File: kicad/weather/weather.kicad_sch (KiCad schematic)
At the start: 6 parts

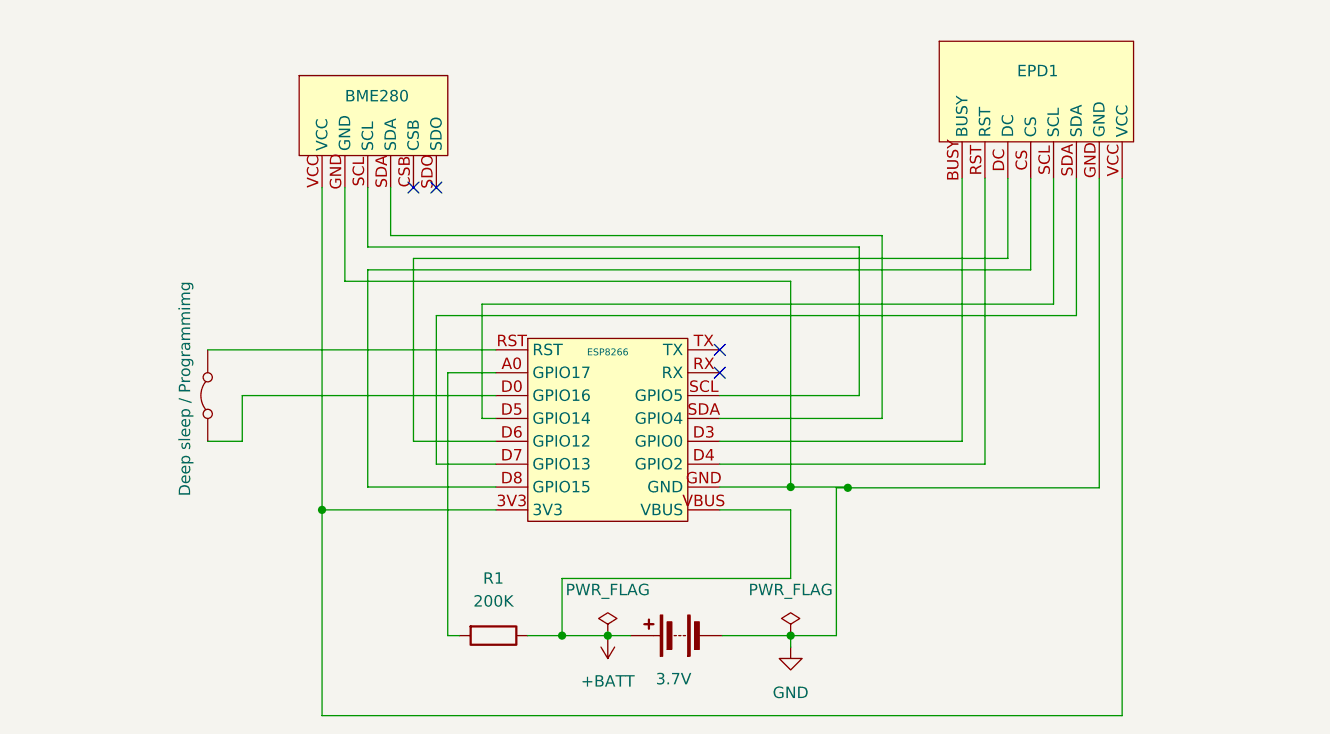
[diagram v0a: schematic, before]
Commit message: Finalized schematics and PCB
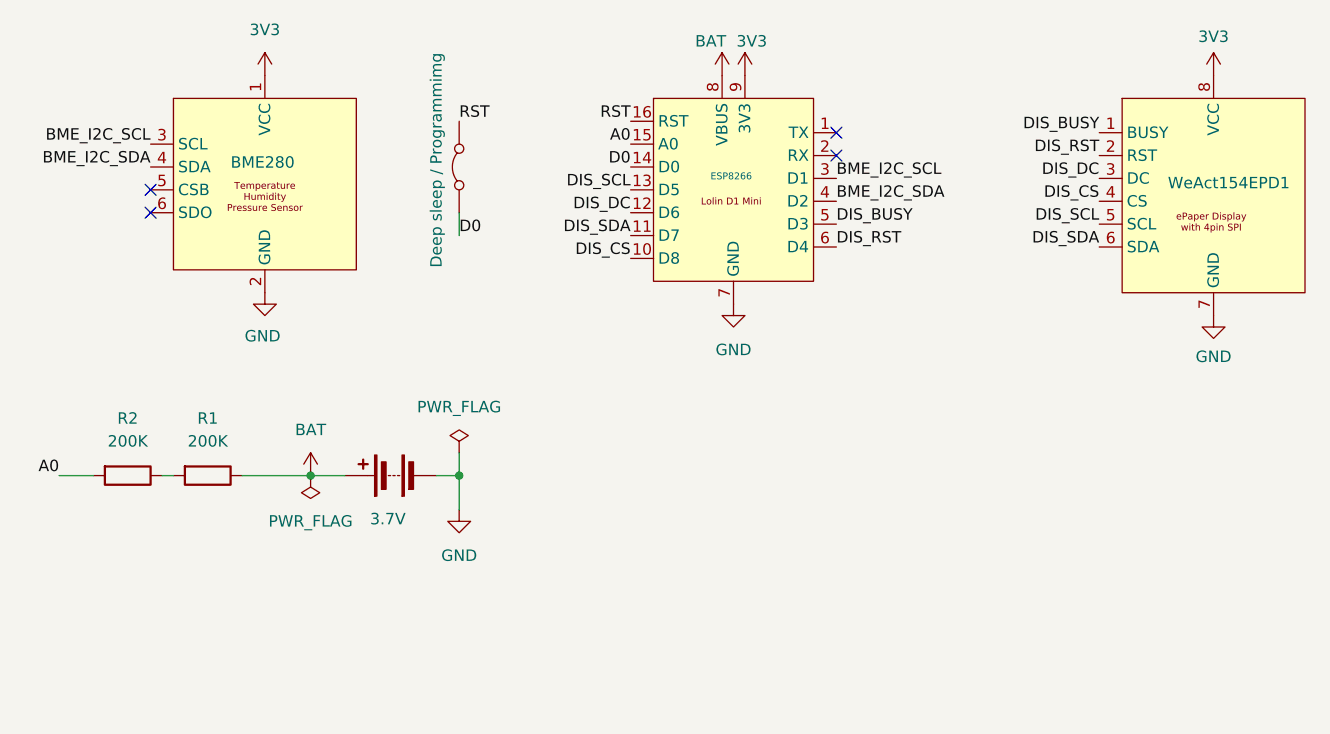
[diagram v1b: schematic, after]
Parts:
- added R2: 200K, custom_footprints:4er DIP, symbol Device:R
- BME280: footprint (none) -> custom_footprints:BME280 DIP
- BT_18650: footprint (none) -> Connector_JST:JST_EH_B2B-EH-A_1x02_P2.50mm_Vertical
- ESP8266: footprint (none) -> custom_footprints:LOLIN D1 MINI DIP
- JP1: footprint (none) -> custom_footprints:2er DIP
- R1: footprint (none) -> custom_footprints:4er DIP
- WeAct154EPD1: renamed from EPD1; footprint (none) -> custom_footprints:1,54 EPD SPI DIP
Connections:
- net GND: now also BME280.2 (GND), ESP8266.7 (GND), WeAct154EPD1.7 (GND); no longer BME280.GND, ESP8266.GND, WeAct154EPD1.GND
- net at R1.2: now also R2.1; no longer ESP8266.A0 (GPIO17)
- net D0: now reaches JP1.1 (A)
- net D0: now also ESP8266.14 (D0); no longer ESP8266.D0 (GPIO16)
- net RST: now reaches JP1.2 (B)
- net RST: now also ESP8266.16 (RST); no longer ESP8266.RST
- net +BATT renamed BAT
- net BAT: now also ESP8266.8 (VBUS); no longer ESP8266.VBUS
- new net 3V3: BME280.1 (VCC), ESP8266.9 (3V3), WeAct154EPD1.8 (VCC)
- new net A0: ESP8266.15 (A0), R2.2
- new net BME_I2C_SCL: BME280.3 (SCL), ESP8266.3 (D1)
- new net BME_I2C_SDA: BME280.4 (SDA), ESP8266.4 (D2)
- new net DIS_BUSY: ESP8266.5 (D3), WeAct154EPD1.1 (BUSY)
- new net DIS_CS: ESP8266.10 (D8), WeAct154EPD1.4 (CS)
- new net DIS_DC: ESP8266.12 (D6), WeAct154EPD1.3 (DC)
- new net DIS_RST: ESP8266.6 (D4), WeAct154EPD1.2 (RST)
- new net DIS_SCL: ESP8266.13 (D5), WeAct154EPD1.5 (SCL)
- new net DIS_SDA: ESP8266.11 (D7), WeAct154EPD1.6 (SDA)
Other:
- moved on the sheet: R1
